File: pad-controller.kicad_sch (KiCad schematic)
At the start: 21 parts, among them J1 Conn_01x02, J3 Conn_01x02, J6 Conn_01x06, M1 Motor_Servo, M2 Motor_Servo, M3 Motor_Servo, M4 Motor_Servo, Q1 IRFP450PBF, Q2 FQP30N06L, SW1 SW_Push_Dual, U1 Xbee

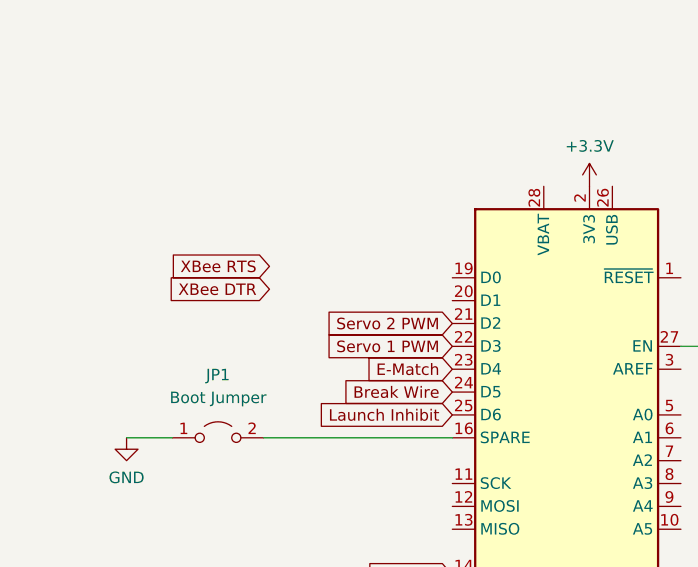
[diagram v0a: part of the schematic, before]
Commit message: Adjust layout
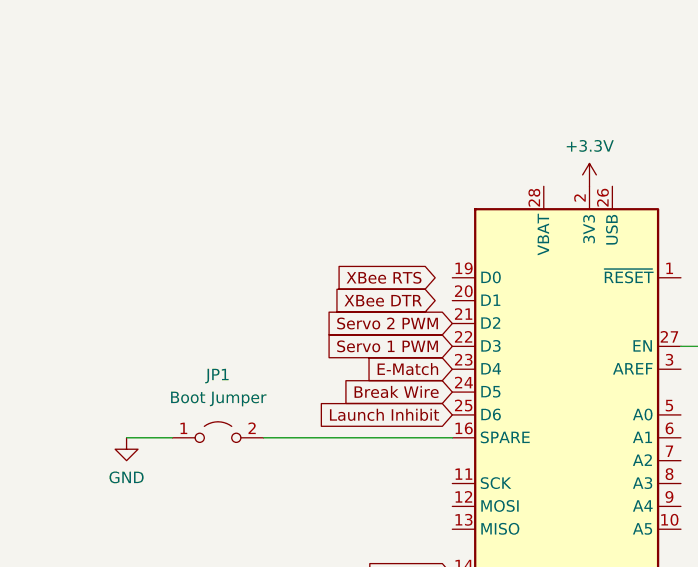
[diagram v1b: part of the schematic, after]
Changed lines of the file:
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@@
     )
   )
-  (global_label "XBee RTS" (shape input) (at 45.72 51.435 180) (fields_autoplaced)
+  (global_label "XBee RTS" (shape input) (at 64.135 52.705 180) (fields_autoplaced)
     (effects (font (size 1.27 1.27)) (justify right))
-    (property "Intersheetrefs" "${INTERSHEET_REFS}" (at 33.6634 51.435 0)
+    (property "Intersheetrefs" "${INTERSHEET_REFS}" (at 52.0784 52.705 0)
       (effects (font (size 1.27 1.27)) (justify right) hide)
     )
@@
     )
   )
-  (global_label "XBee DTR" (shape input) (at 45.72 53.975 180) (fields_autoplaced)
+  (global_label "XBee DTR" (shape input) (at 64.135 55.245 180) (fields_autoplaced)
     (effects (font (size 1.27 1.27)) (justify right))
-    (property "Intersheetrefs" "${INTERSHEET_REFS}" (at 33.6029 53.975 0)
+    (property "Intersheetrefs" "${INTERSHEET_REFS}" (at 52.0179 55.245 0)
       (effects (font (size 1.27 1.27)) (justify right) hide)
     )
